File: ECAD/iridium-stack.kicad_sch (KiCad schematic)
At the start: 13 parts

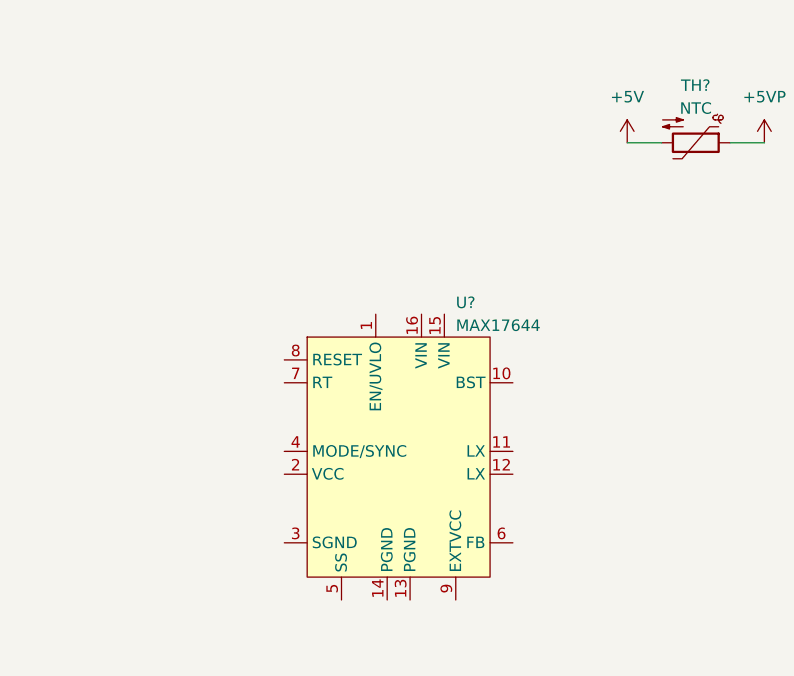
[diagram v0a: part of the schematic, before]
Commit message: ap62301
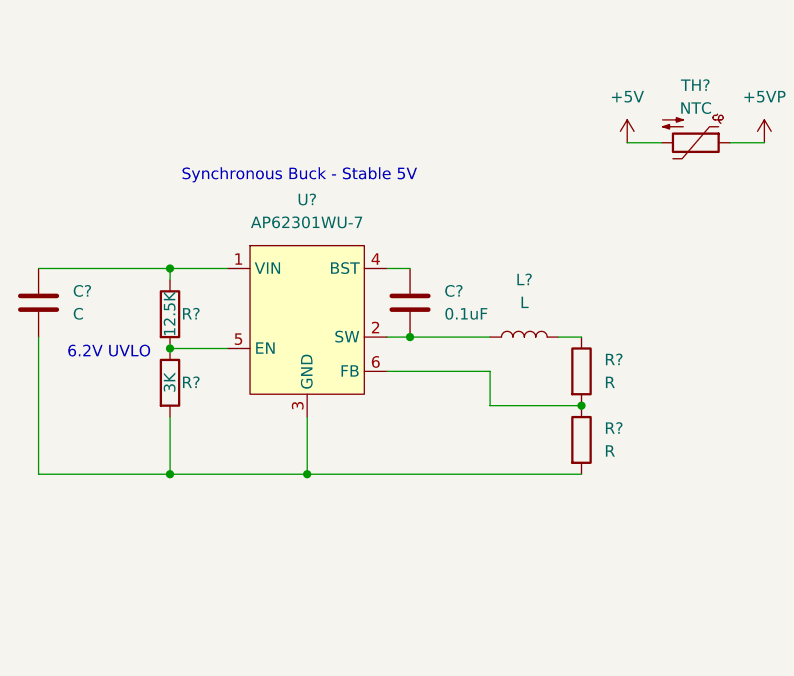
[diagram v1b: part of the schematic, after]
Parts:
- removed U?: MAX17644, symbol Symbols:MAX17644
- added C?: 0.1uF, symbol Device:C
- added C?: C, symbol Device:C
- added L?: L, symbol Device:L
- added R? (x2): R, symbol Device:R
- added R?: 3K, symbol Device:R
- added R?: 12.5K, symbol Device:R
- added U?: AP62301WU-7, symbol Symbols:AP62301WU-7
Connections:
- new net: R?.1, R?.2, U?.6 (FB)
- new net: C?.2, R?.2, R?.2, U?.3 (GND)
- new net: C?.1, U?.4 (BST)
- new net: C?.2, L?.1, U?.2 (SW)
- new net: C?.1, R?.1, U?.1 (VIN)
- new net: R?.1, R?.2, U?.5 (EN)
- new net: L?.2, R?.1
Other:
- note added: "6.2V UVLO"
- note added: "Synchronous Buck - Stable 5V"
